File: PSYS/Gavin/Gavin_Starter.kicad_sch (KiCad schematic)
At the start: 41 parts, among them J1 Conn_Coaxial, J2 Conn_ARM_SWD_TagConnect_TC2030, J3 USB_C_Receptacle_USB2.0_16P, J4 Conn_01x04, SW1 SW_Push, U1 STM32WB55CEUx, U2 USBLC6-2SC6, U3 MIC5365-3.3YD5, X1 32MHz, X2 32Khz768

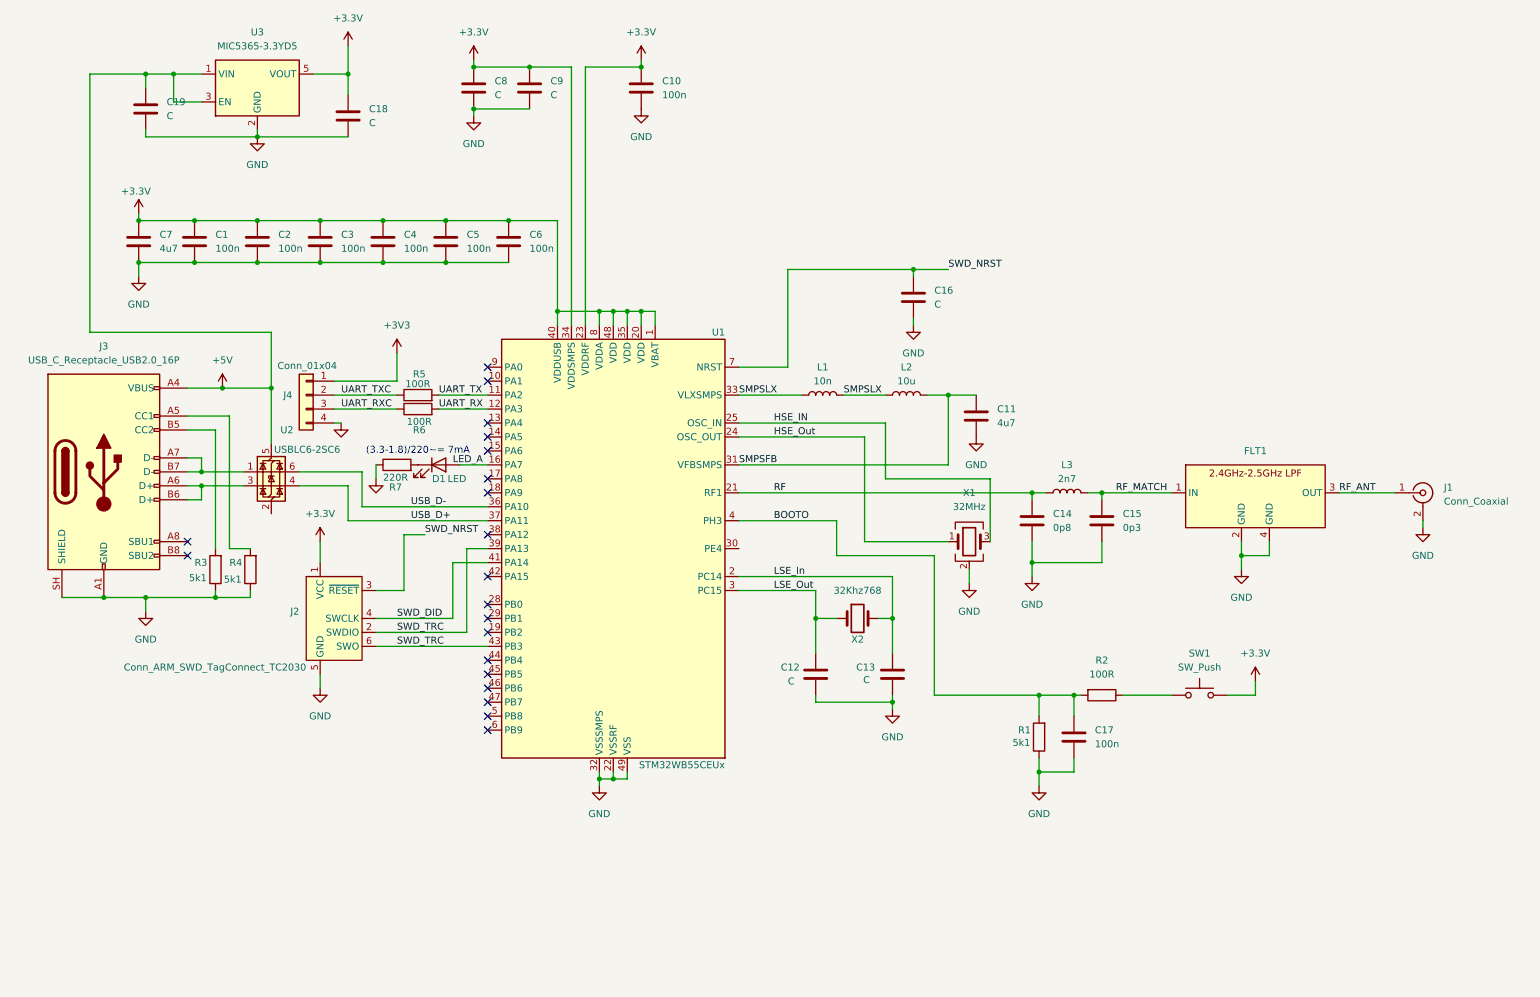
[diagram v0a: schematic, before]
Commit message: schematic2
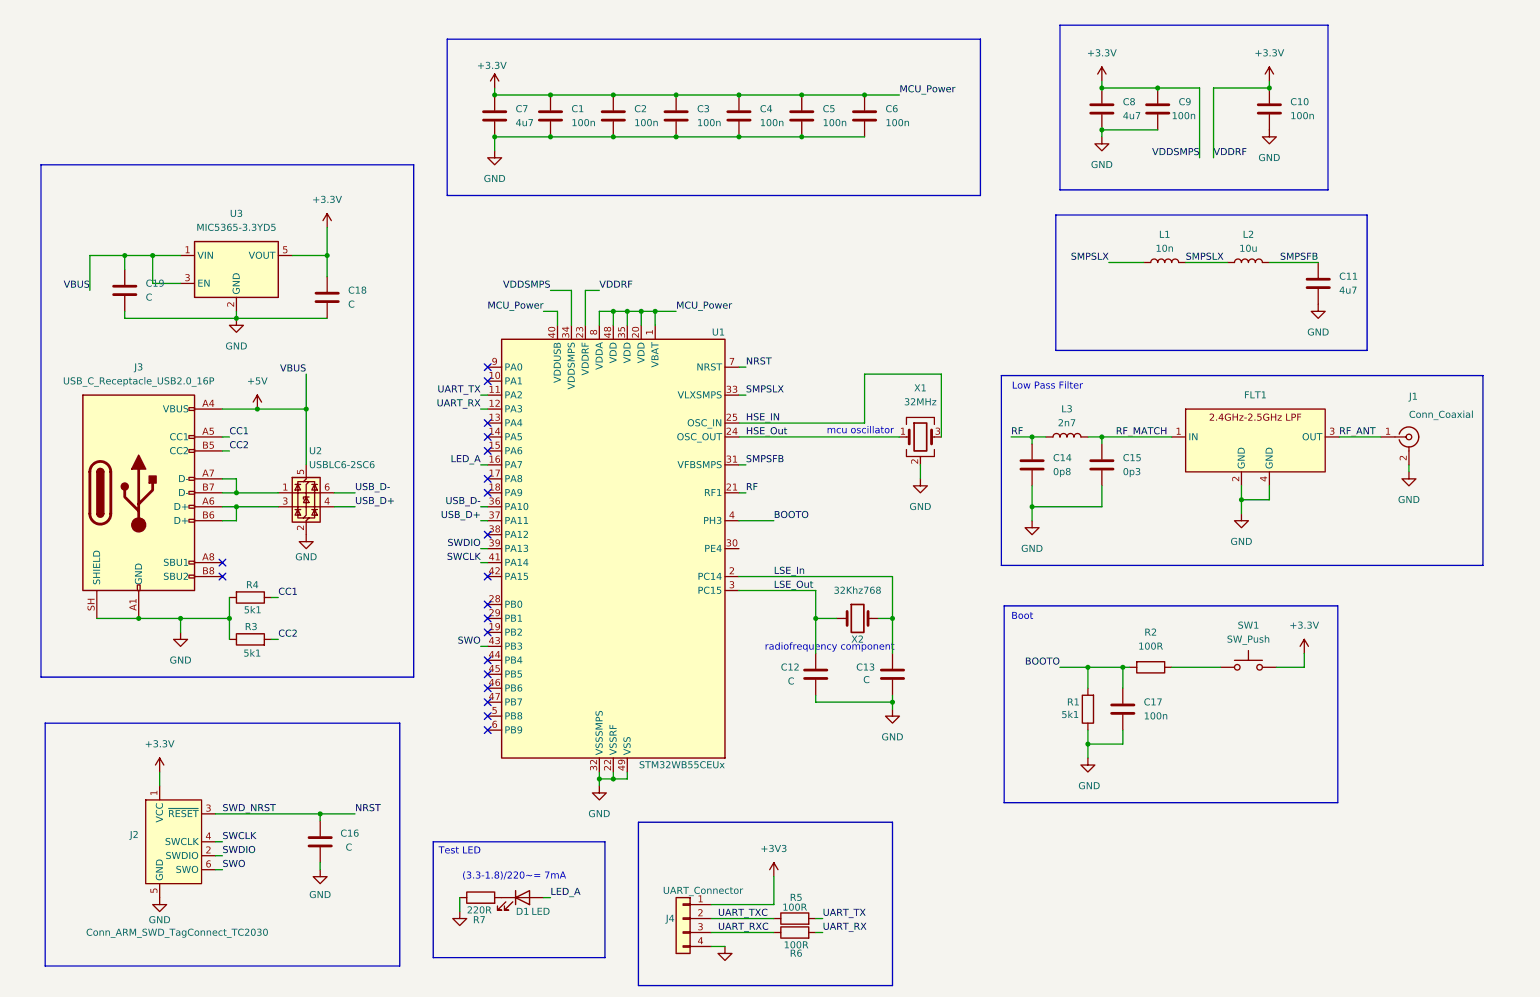
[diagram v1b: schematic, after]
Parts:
- C8: value C -> 4u7
- C9: value C -> 100n
- J4: value Conn_01x04 -> UART_Connector
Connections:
- net GND: now also R4.2, U2.2 (GND); no longer R4.1
- net LED_A: now also D1.2 (A), U1.16 (PA7)
- net CC2: now reaches J3.B5 (CC2), R3.2
- net CC1: now reaches J3.A5 (CC1)
- net CC1: now also R4.1; no longer R4.2
- net SWD_DID renamed SWCLK
- net SWD_NRST renamed NRST
- net SWD_TRC renamed SWDIO
- net SWDIO: no longer J2.6 (SWO), U1.43 (PB3)
- new net SWO: J2.6 (SWO), U1.43 (PB3)
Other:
- note added: "Boot"
- note added: "Low Pass Filter"
- note added: "Test LED"
- note added: "mcu oscillator"
- note added: "radiofrequency component"
- moved on the sheet: C1, C10, C11, C14, C15, C16, C17, C18, C19, C2, C3, C4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
